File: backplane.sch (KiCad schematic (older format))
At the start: 29 parts, among them J1 I2C, J2 I2C, J3 SER, J4 PWR, J5 PWR, J6 FAN, Q1 Q_NMOS_DGS, Q2 Q_NMOS_DGS, Q3 Q_NMOS_DGS, Q4 Q_NMOS_DGS, U1 Raspberry_Pi_2_3, U2 IC880A-SPI, U3 SHT21, U4 MP1584_MODULE

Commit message: Fix NMOS parts in schema
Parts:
- Q1, Q2, Q3, Q4: value Q_NMOS_DGS -> Q_NMOS_GSD; symbol Q_NMOS_DGS -> Q_NMOS_GSD
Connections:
- wire segments 170 -> 169
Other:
- moved on the sheet: D1, D3, R1, R3, R6, R7, R8

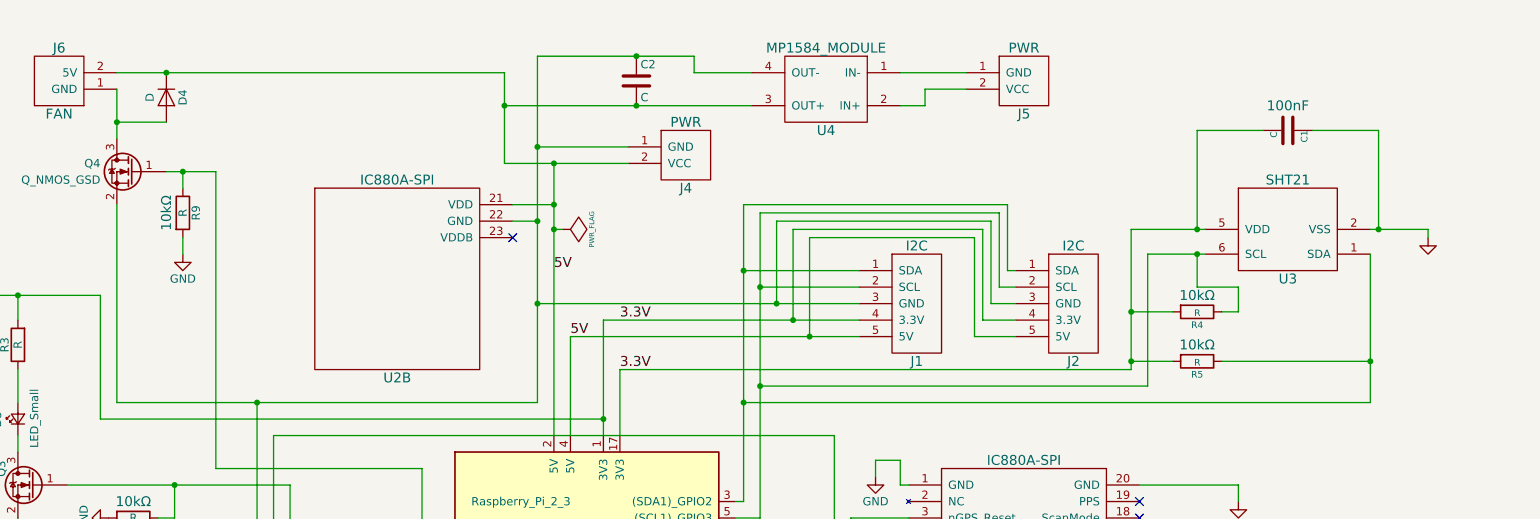
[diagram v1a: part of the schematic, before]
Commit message: Start splitting up schema with labels
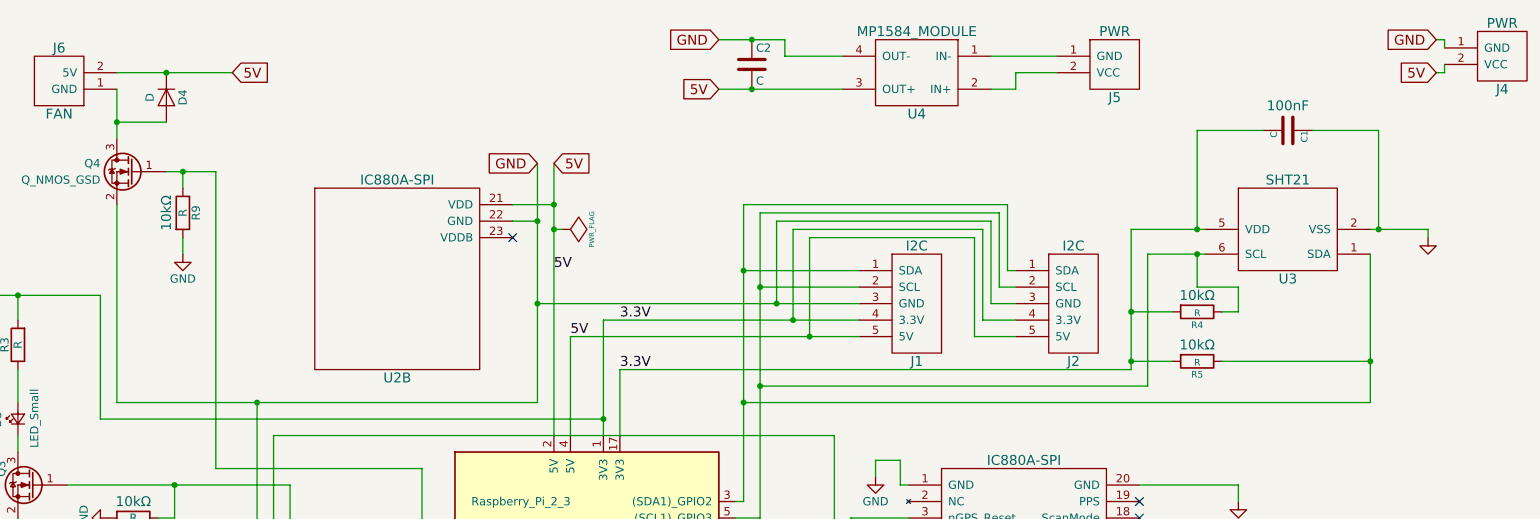
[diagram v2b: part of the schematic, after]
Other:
- moved on the sheet: C2, J4, J5, U4
